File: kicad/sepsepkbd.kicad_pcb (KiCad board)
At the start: 2 copper layers, 142.4 x 134.1 mm, 47 parts, among them J1 MJ-4PP-9, J2 Conn_01x04_Socket, J3 Conn_01x04_Socket, SW1 SW_PUSH, SW10 SW_PUSH, SW11 SW_PUSH, SW12 SW_PUSH, SW13 SW_PUSH, SW14 SW_PUSH, SW15 SW_PUSH, SW16 SW_PUSH, SW17 SW_PUSH, SW18 SW_PUSH, SW19 SW_PUSH, SW2 SW_PUSH, SW20 SW_PUSH, SW21 SW_PUSH, SW3 SW_PUSH, SW4 SW_PUSH, SW5 SW_PUSH, SW6 SW_PUSH, SW7 SW_PUSH, SW8 SW_PUSH, SW9 SW_PUSH, U1 ProMicro

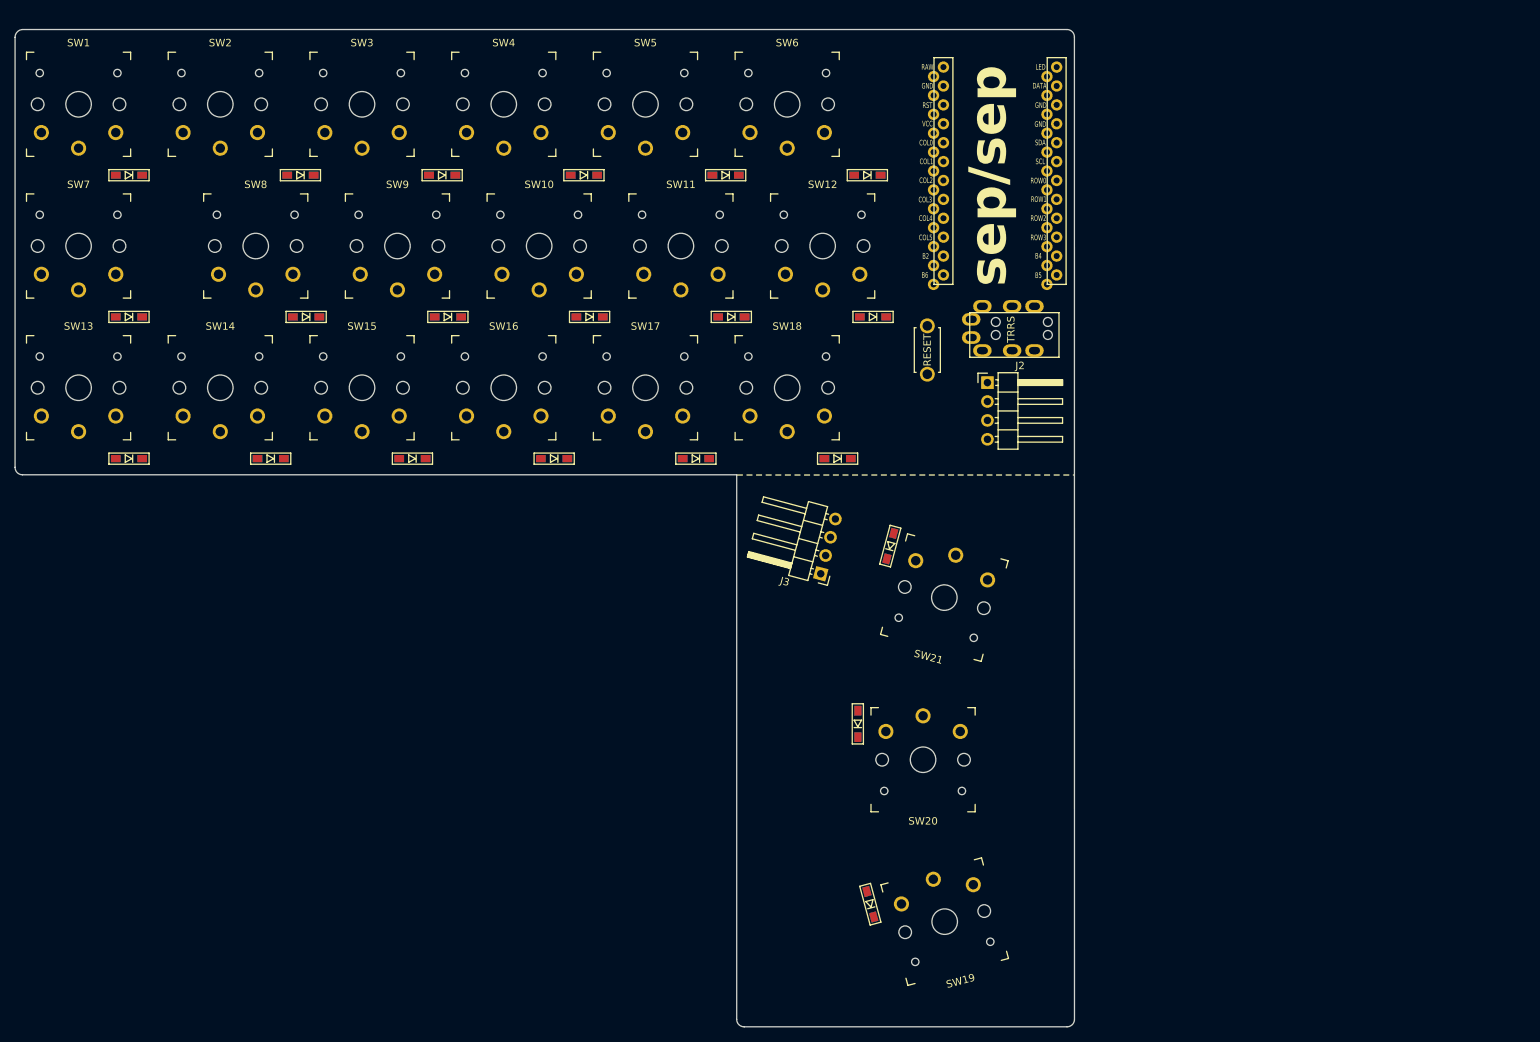
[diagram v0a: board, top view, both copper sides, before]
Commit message: add boy's heart
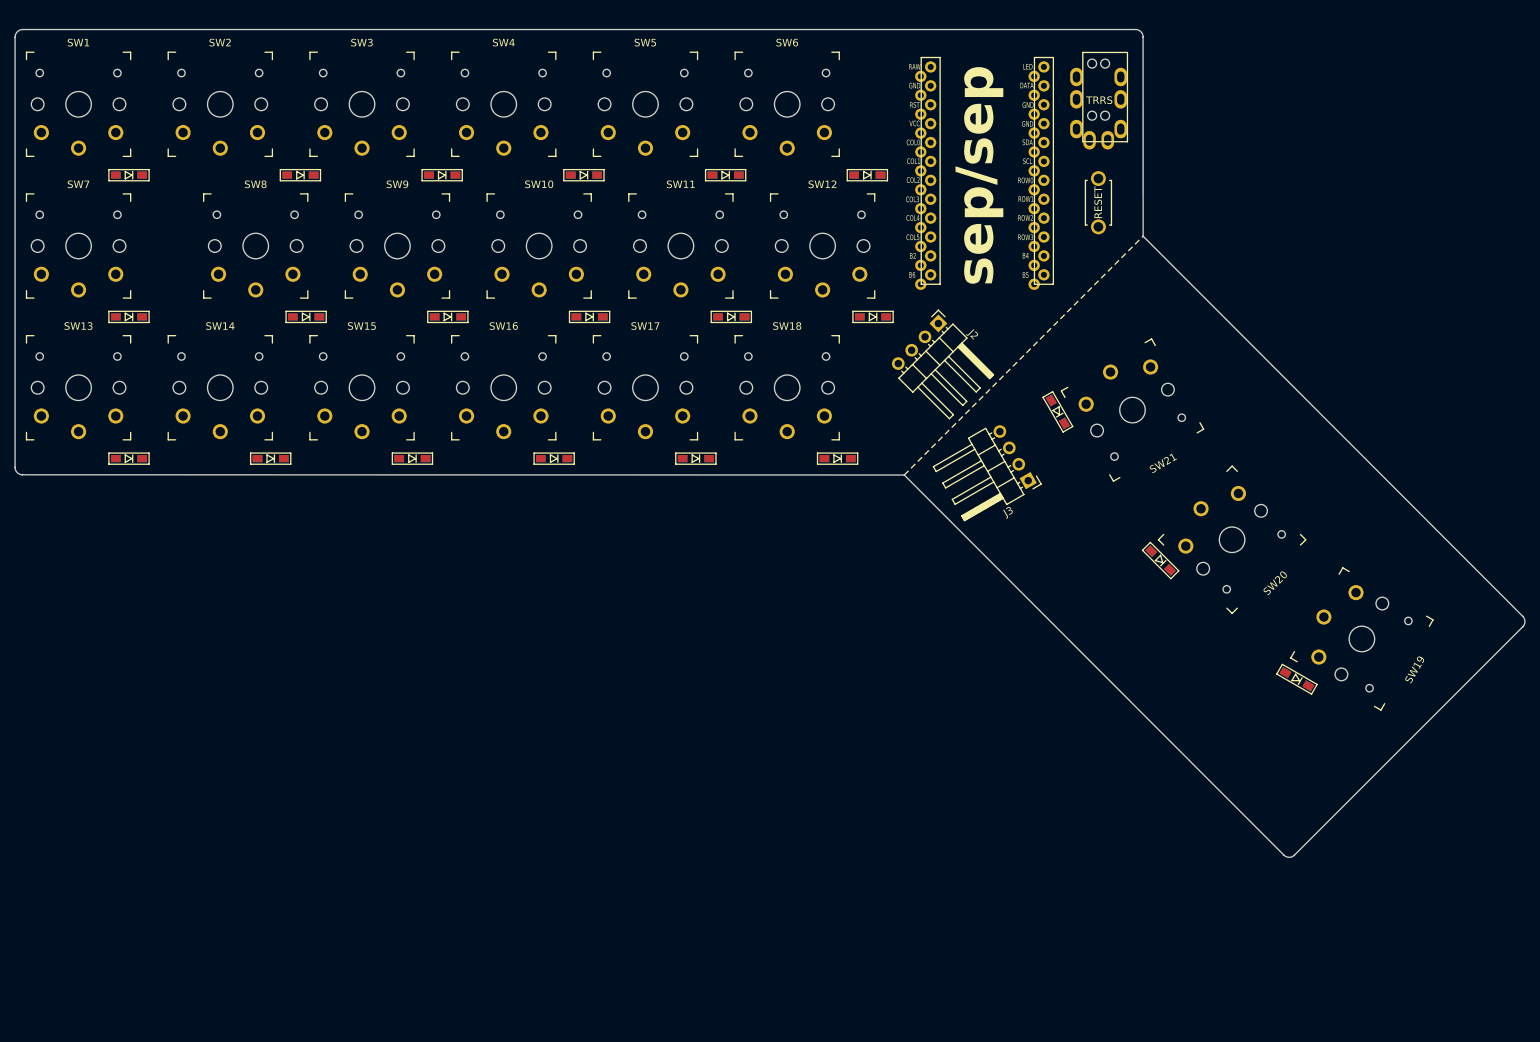
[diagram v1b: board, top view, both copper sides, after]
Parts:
- moved SW19 67.7 mm to (208.3, 118.9), turned to -120 degrees
- moved D19 64.8 mm to (199.6, 124.4), turned to 150 degrees
- moved SW20 51.0 mm to (190.9, 105.6), turned to -135 degrees
- moved D20 46.2 mm to (181.3, 108.4), turned to 135 degrees
- moved J1 38.5 mm to (173.8, 40.1), turned to 0 degrees
- moved SW21 35.7 mm to (177.5, 88.2), turned to -150 degrees
- moved J3 30.6 mm to (163.5, 97.7), turned to -150 degrees
- moved SW_RESET1 30.3 mm to (172.9, 60.3), turned to -90 degrees
- moved D21 28.9 mm to (167.4, 88.4), turned to 120 degrees
- moved J2 10.3 mm to (151.4, 76.5), turned to -45 degrees
- moved U1 1.72 mm to (157.9, 56.5)
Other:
- board size 142.4 x 134.1 mm -> 202.9 x 111.3 mm
